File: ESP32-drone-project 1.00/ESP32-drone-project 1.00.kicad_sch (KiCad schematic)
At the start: 2 parts

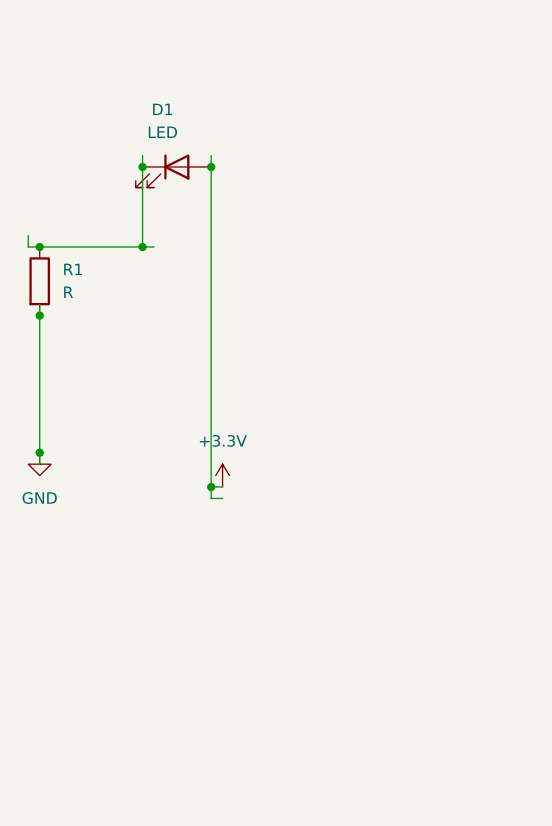
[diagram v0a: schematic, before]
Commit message: Add files via upload
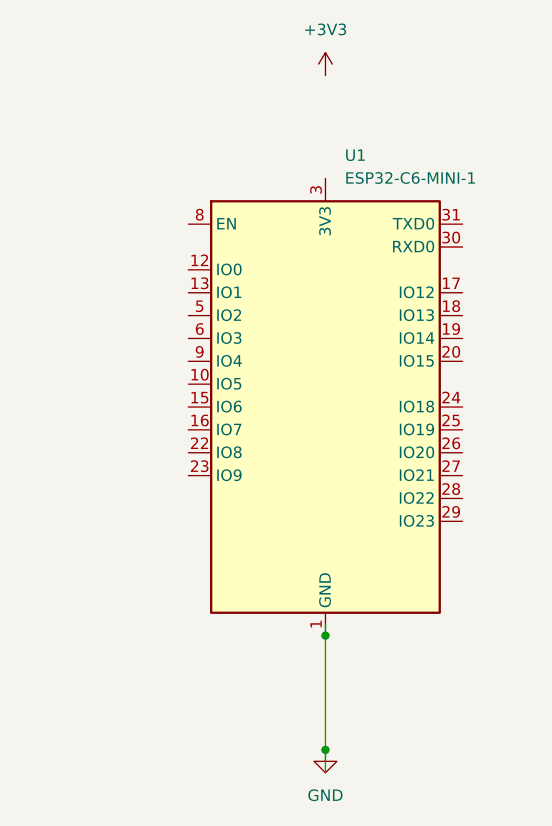
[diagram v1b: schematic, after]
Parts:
- removed D1: LED, symbol Device:LED
- removed R1: R, symbol Device:R
- added U1: ESP32-C6-MINI-1, RF_Module:ESP32-C6-MINI-1, symbol RF_Module:ESP32-C6-MINI-1
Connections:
- net GND: now also U1.1 (GND), U1.11 (GND), U1.14 (GND), U1.2 (GND), U1.36 (GND), U1.37 (GND), U1.38 (GND), U1.39 (GND), U1.40 (GND), U1.41 (GND), U1.42 (GND), U1.43 (GND), U1.44 (GND), U1.45 (GND), U1.46 (GND), U1.47 (GND), U1.48 (GND), U1.49 (GND), U1.50 (GND), U1.51 (GND), U1.52 (GND), U1.53 (GND)
